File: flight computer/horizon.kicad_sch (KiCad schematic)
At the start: 44 parts, among them J2 Conn_02x03_Counter_Clockwise, J7 Conn_02x03_Counter_Clockwise, J8 Conn_02x03_Counter_Clockwise, SW1 CK_KMS2xxG, U1 MMCU, U2 MKL02Z32VFG4, Y1 Crystal

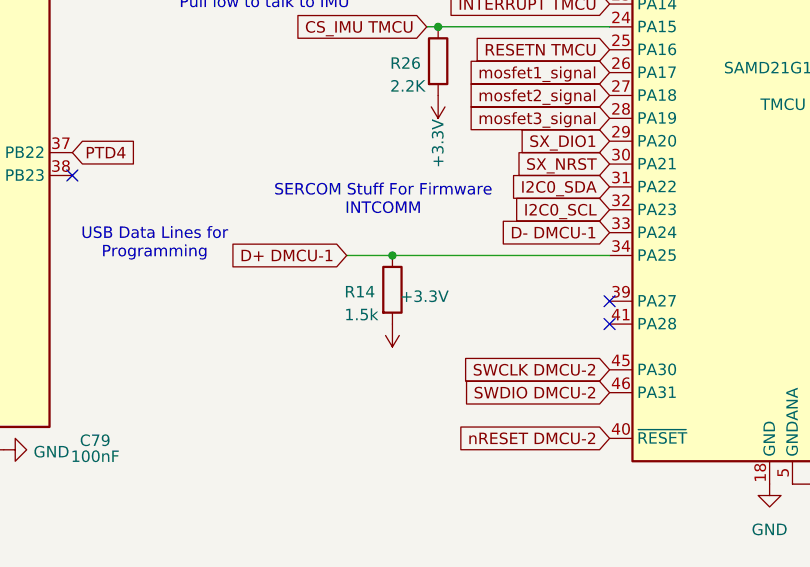
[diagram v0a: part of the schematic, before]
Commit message: force push :'/
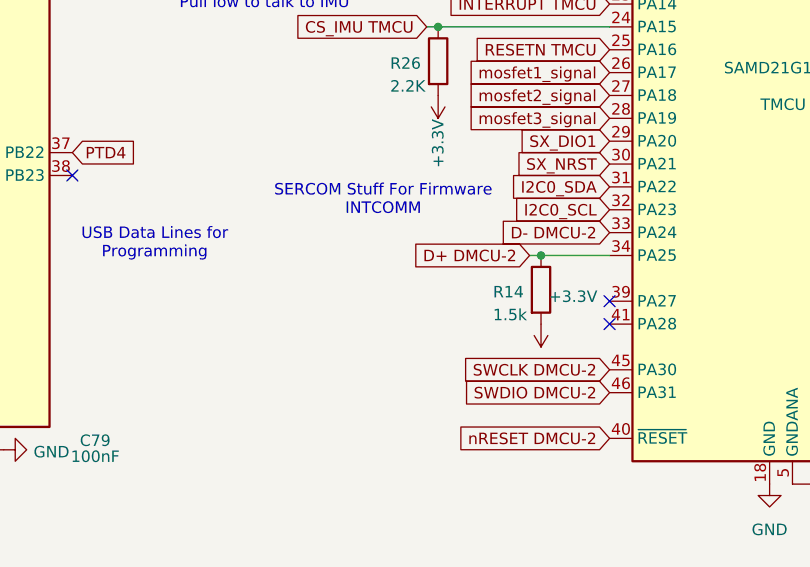
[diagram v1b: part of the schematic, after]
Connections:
- net D+ DMCU-1: no longer R14.1, SAMD21G18A-AU2.34 (PA25)
- net D- DMCU-1: no longer SAMD21G18A-AU2.33 (PA24)
- new net D+ DMCU-2: R14.1, SAMD21G18A-AU2.34 (PA25)
- new net D- DMCU-2: SAMD21G18A-AU2.33 (PA24)
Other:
- moved on the sheet: R14
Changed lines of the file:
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@@
 	)
 	(junction
-		(at 102.87 107.95)
-		(diameter 0)
-		(color 0 0 0 0)
-	)
-	(junction
 		(at 224.79 93.98)
 		(diameter 0)
@@
 	)
 	(junction
+		(at 119.38 107.95)
+		(diameter 0)
+		(color 0 0 0 0)
+	)
+	(junction
 		(at 209.55 133.35)
 		(diameter 0)
@@
 	(wire
 		(pts
+			(xy 119.38 107.95) (xy 127 107.95)
+		)
+		(stroke
+			(width 0)
+			(type default)
+		)
+	)
+	(wire
+		(pts
 			(xy 384.81 118.11) (xy 384.81 115.57)
 		)
@@
 	(wire
 		(pts
-			(xy 97.79 107.95) (xy 102.87 107.95)
+			(xy 118.11 107.95) (xy 119.38 107.95)
 		)
 		(stroke
@@
 	(wire
 		(pts
-			(xy 102.87 107.95) (xy 127 107.95)
-		)
-		(stroke
-			(width 0)
-			(type default)
-		)
-	)
-	(wire
-		(pts
 			(xy 383.54 118.11) (xy 384.81 118.11)
 		)
@@
 		)
 	)
-	(global_label "D+ DMCU-1"
+	(global_label "D+ DMCU-2"
 		(shape input)
-		(at 97.79 107.95 180)
+		(at 118.11 107.95 180)
 		(fields_autoplaced yes)
 		(effects
@@
 		)
 		(property "Intersheetrefs" "${INTERSHEET_REFS}"
-			(at 82.891 107.95 0)
+			(at 103.211 107.95 0)
 			(effects
 				(font
@@
 		)
 	)
-	(global_label "D- DMCU-1"
+	(global_label "D- DMCU-2"
 		(shape input)
 		(at 127 105.41 180)
@@
 	(symbol
 		(lib_id "power:+3.3V")
-		(at 102.87 115.57 180)
+		(at 119.38 115.57 180)
 		(unit 1)
 		(exclude_from_sim no)
@@
 		(dnp no)
 		(property "Reference" "#PWR037"
-			(at 102.87 111.76 0)
+			(at 119.38 111.76 0)
 			(effects
 				(font
@@
 		)
 		(property "Value" "+3.3V"
-			(at 106.426 112.522 0)
+			(at 122.936 112.522 0)
 			(effects
 				(font
@@
 		)
 		(property "Footprint" ""
-			(at 102.87 115.57 0)
+			(at 119.38 115.57 0)
 			(effects
 				(font
@@
 		)
 		(property "Datasheet" ""
-			(at 102.87 115.57 0)
+			(at 119.38 115.57 0)
 			(effects
 				(font
@@
 		)
 		(property "Description" "Power symbol creates a global label with name \"+3.3V\""
-			(at 102.87 115.57 0)
+			(at 119.38 115.57 0)
 			(effects
 				(font
@@
 	(symbol
 		(lib_id "Device:R")
-		(at 102.87 111.76 0)
+		(at 119.38 111.76 0)
 		(unit 1)
 		(exclude_from_sim no)
@@
 		(dnp no)
 		(property "Reference" "R14"
-			(at 97.536 112.014 0)
+			(at 114.046 112.014 0)
 			(effects
 				(font
@@
 		)
 		(property "Value" "1.5k"
-			(at 97.536 114.554 0)
+			(at 114.046 114.554 0)
 			(effects
 				(font
@@
 		)
 		(property "Footprint" "Resistor_SMD:R_0603_1608Metric"
-			(at 101.092 111.76 90)
+			(at 117.602 111.76 90)
 			(effects
 				(font
@@
 		)
 		(property "Datasheet" "~"
-			(at 102.87 111.76 0)
+			(at 119.38 111.76 0)
 			(effects
 				(font
@@
 		)
 		(property "Description" "Resistor"
-			(at 102.87 111.76 0)
+			(at 119.38 111.76 0)
 			(effects
 				(font
